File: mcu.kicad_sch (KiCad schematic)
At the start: 10 parts, among them J37 Micro_SD_Card, J38 Micro_SD_Card

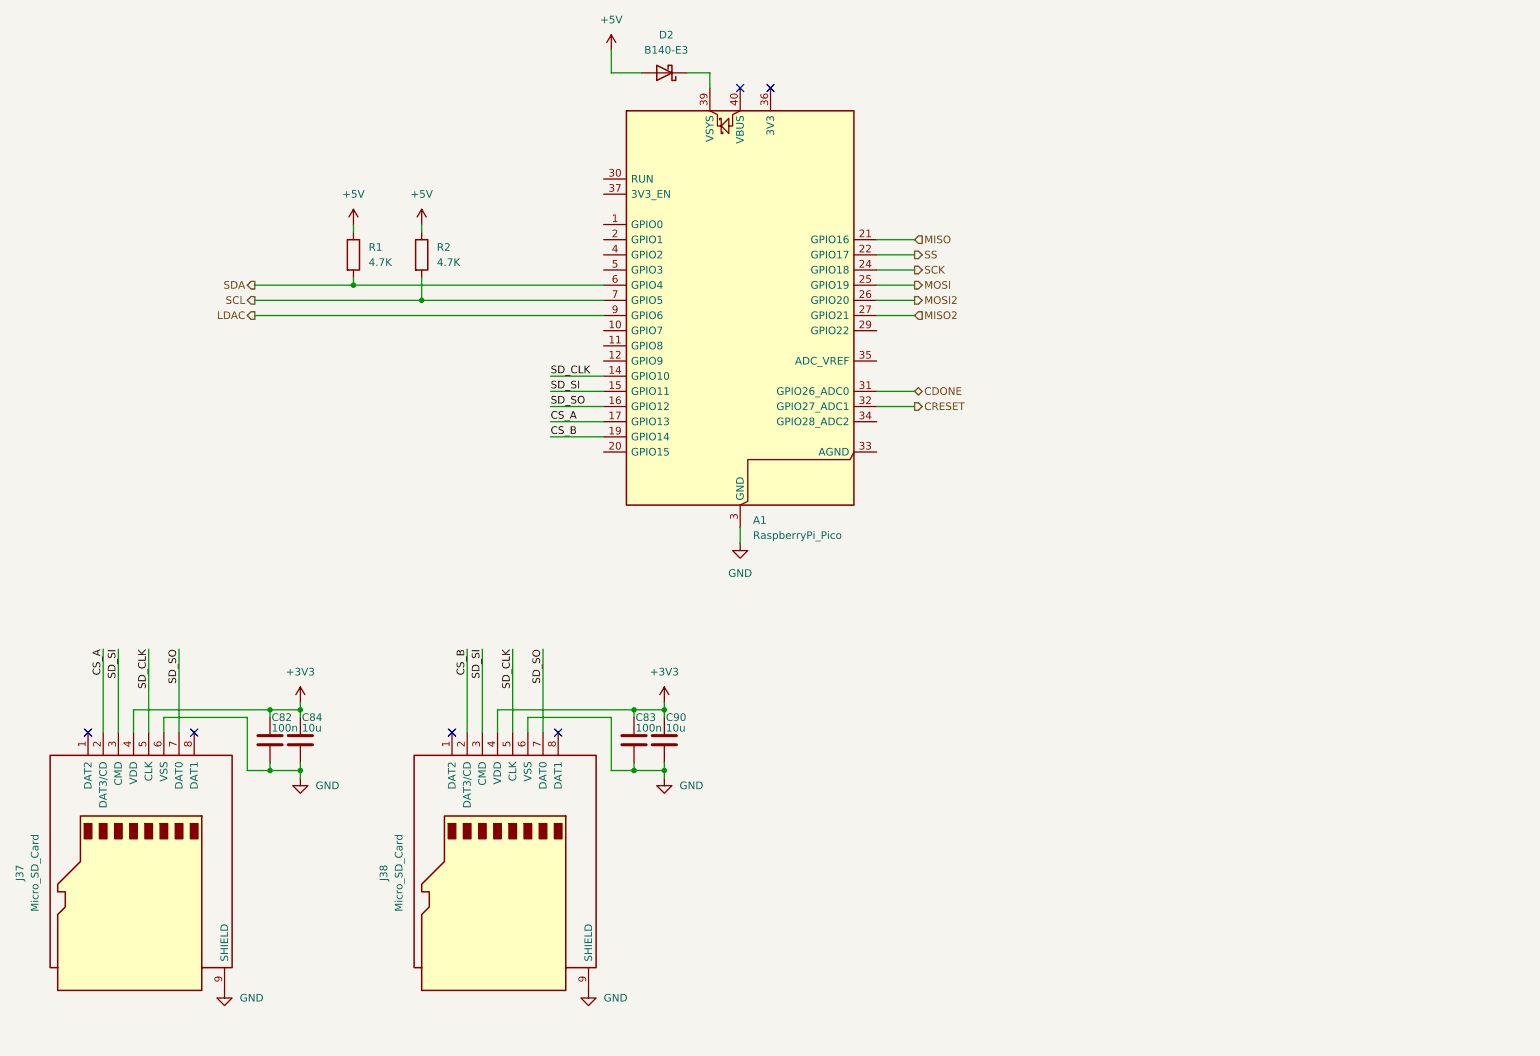
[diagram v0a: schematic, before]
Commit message: rewire
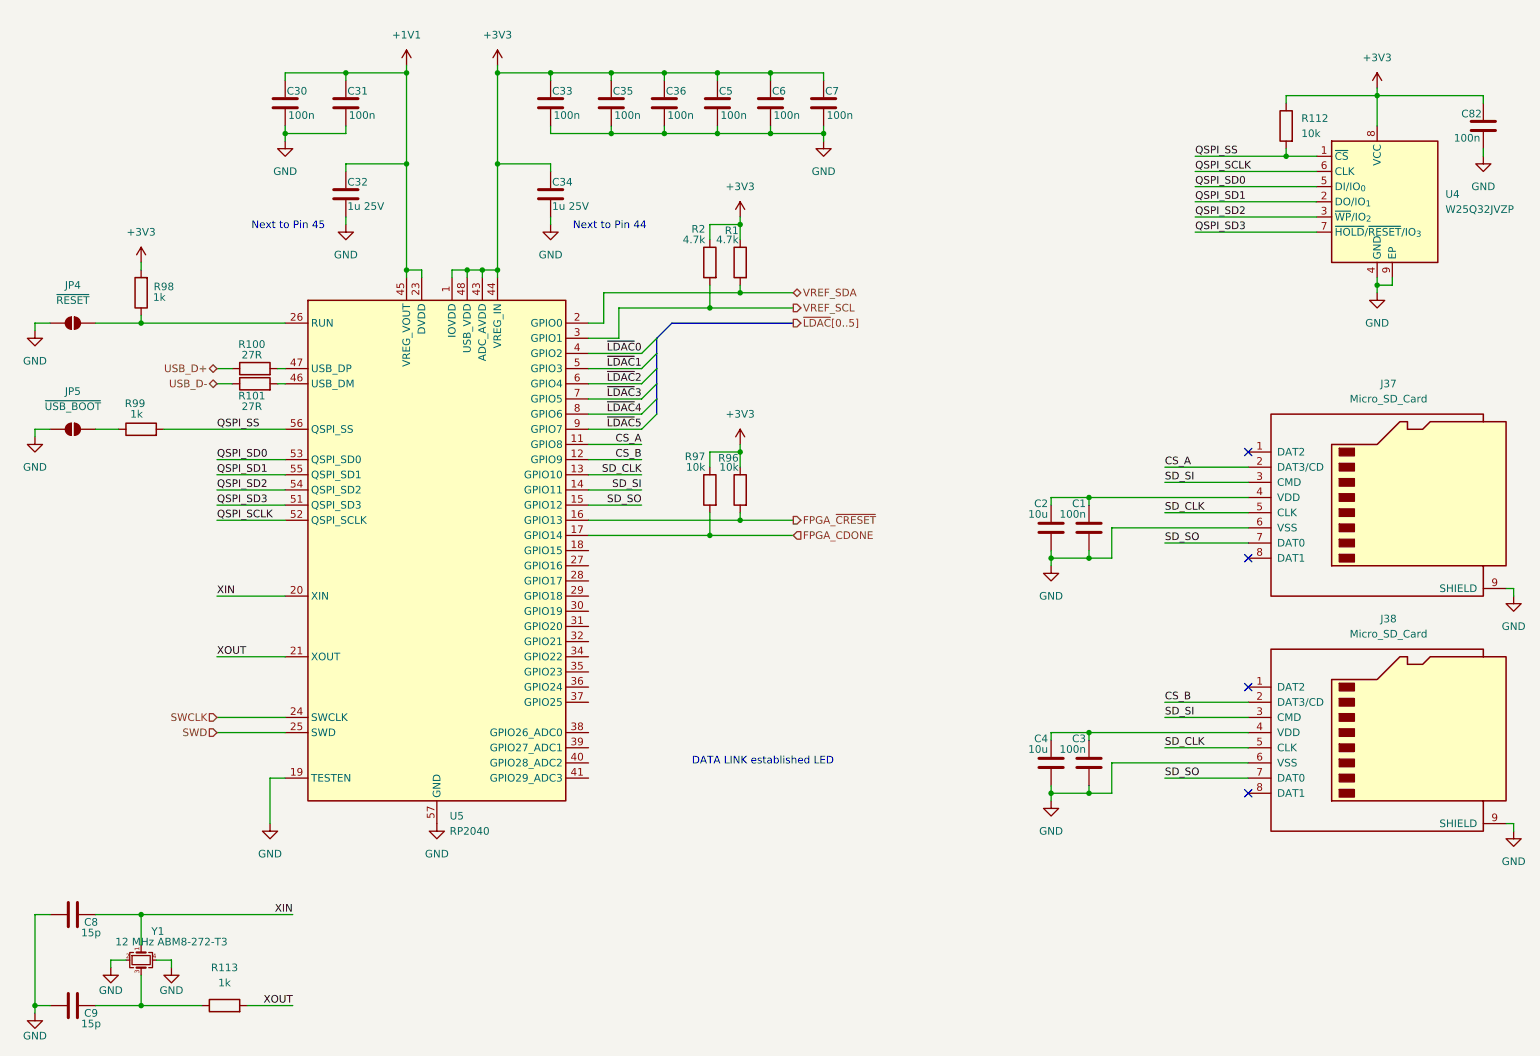
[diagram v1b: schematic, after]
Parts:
- removed A1: RaspberryPi_Pico, Module:RaspberryPi_Pico_Common_Unspecified, symbol MCU_Module:RaspberryPi_Pico
- removed C83: 100n, symbol Device:C
- removed C84, C90: 10u, symbol Device:C
- removed D2: B140-E3, symbol Device:D_Schottky
- added C1, C3: 100n, symbol Device:C
- added C2, C4: 10u, symbol Device:C
- added C30, C31, C33, C35, C36, C5, C6, C7: 100n, Capacitor_SMD:C_0402_1005Metric, symbol Device:C
- added C32, C34: 1u 25V, Capacitor_SMD:C_0402_1005Metric, symbol Device:C
- added C8, C9: 15p, Capacitor_SMD:C_0402_1005Metric, symbol Device:C
- added JP4: ~{RESET}, Jumper:SolderJumper-2_P1.3mm_Open_RoundedPad1.0x1.5mm, symbol Jumper:SolderJumper_2_Open
- added JP5: ~{USB_BOOT}, Jumper:SolderJumper-2_P1.3mm_Open_RoundedPad1.0x1.5mm, symbol Jumper:SolderJumper_2_Open
- added R100, R101: 27R, Resistor_SMD:R_0402_1005Metric, symbol Device:R
- added R112: 10k, Resistor_SMD:R_0402_1005Metric, symbol Device:R
- added R113, R98, R99: 1k, Resistor_SMD:R_0402_1005Metric, symbol Device:R
- added R96, R97: 10k, symbol Device:R
- added U4: W25Q32JVZP, Package_SON:WSON-8-1EP_6x5mm_P1.27mm_EP3.4x4.3mm, symbol Memory_Flash:W25Q32JVZP
- added U5: RP2040, Package_DFN_QFN:QFN-56-1EP_7x7mm_P0.4mm_EP3.2x3.2mm, symbol MCU_RaspberryPi:RP2040
- added Y1: 12 MHz ABM8-272-T3, Crystal:Crystal_SMD_Abracon_ABM8AIG-4Pin_3.2x2.5mm, symbol Device:Crystal_GND24_Small
- C82: footprint (none) -> Capacitor_SMD:C_0402_1005Metric; LCSC (none) -> C307331
- R1, R2: value 4.7K -> 4.7k
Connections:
- net +5V is gone; now on net +3V3: R1.1, R2.1
- net +3V3: now also C33.1, C34.1, C35.1, C36.1, C5.1, C6.1, C7.1, R112.1, R96.1, R97.1, R98.2, U4.8 (VCC), U5.1 (IOVDD), U5.10 (IOVDD), U5.22 (IOVDD), U5.33 (IOVDD), U5.42 (IOVDD), U5.43 (ADC_AVDD), U5.44 (VREG_IN), U5.48 (USB_VDD), U5.49 (IOVDD); no longer J37.4 (VDD), J38.4 (VDD)
- net CS_A: now also U5.11 (GPIO8)
- net CS_B: now also U5.12 (GPIO9)
- net GND: now also C1.2, C2.2, C3.2, C30.2, C31.2, C32.2, C33.2, C34.2, C35.2, C36.2, C4.2, C5.2, C6.2, C7.2, C8.1, C9.1, JP4.1 (A), JP5.1 (A), U4.4 (GND), U4.9 (EP), U5.19 (TESTEN), U5.57 (GND), Y1.2, Y1.4
- net SD_CLK: now also U5.13 (GPIO10)
- net SD_SI: now also U5.14 (GPIO11)
- net SD_SO: now also U5.15 (GPIO12)
- net SCL renamed VREF_SCL
- net VREF_SCL: now also U5.3 (GPIO1)
- net SDA renamed VREF_SDA
- net VREF_SDA: now also U5.2 (GPIO0)
- new net: JP4.2 (B), R98.1, U5.26 (RUN)
- new net: JP5.2 (B), R99.1
- new net: R101.2, U5.46 (USB_DM)
- new net: R100.2, U5.47 (USB_DP)
- new net: C9.2, R113.1, Y1.3
- new net: C3.1, C4.1, J38.4 (VDD)
- new net: C1.1, C2.1, J37.4 (VDD)
- new net +1V1: C30.1, C31.1, C32.1, U5.23 (DVDD), U5.45 (VREG_VOUT), U5.50 (DVDD)
- new net FPGA_CDONE: R97.2, U5.17 (GPIO14)
- new net FPGA_~{CRESET}: R96.2, U5.16 (GPIO13)
- new net QSPI_SCLK: U4.6 (CLK), U5.52 (QSPI_SCLK)
- new net QSPI_SD0: U4.5 (DI/IO_{0}), U5.53 (QSPI_SD0)
- new net QSPI_SD1: U4.2 (DO/IO_{1}), U5.55 (QSPI_SD1)
- new net QSPI_SD2: U4.3 (~{WP}/IO_{2}), U5.54 (QSPI_SD2)
- new net QSPI_SD3: U4.7 (~{HOLD}/~{RESET}/IO_{3}), U5.51 (QSPI_SD3)
- new net QSPI_SS: R112.2, R99.2, U4.1 (~{CS}), U5.56 (QSPI_SS)
- new net SWCLK: U5.24 (SWCLK)
- new net SWD: U5.25 (SWD)
- new net USB_D+: R100.1
- new net USB_D-: R101.1
- new net XIN: C8.2, U5.20 (XIN), Y1.1
- new net XOUT: R113.2, U5.21 (XOUT)
- new net ~{LDAC}0: U5.4 (GPIO2)
- new net ~{LDAC}1: U5.5 (GPIO3)
- new net ~{LDAC}2: U5.6 (GPIO4)
- new net ~{LDAC}3: U5.7 (GPIO5)
- new net ~{LDAC}4: U5.8 (GPIO6)
- new net ~{LDAC}5: U5.9 (GPIO7)
- no-connect marks 6 -> 4
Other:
- note added: "DATA LINK established LED"
- note added: "Next to Pin 44"
- note added: "Next to Pin 45"
- moved on the sheet: J37, J38, R1, R2
